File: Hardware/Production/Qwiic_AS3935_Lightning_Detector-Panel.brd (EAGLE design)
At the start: 123.2 x 123.2 mm, 1075 parts, among them U1 AS3935, U10 AS3935, U11 AS3935, U12 AS3935, U13 AS3935, U14 AS3935, U15 AS3935, U16 AS3935, U2 AS3935, U3 AS3935, U4 AS3935, U5 AS3935, U6 AS3935, U7 AS3935, U8 AS3935, U9 AS3935

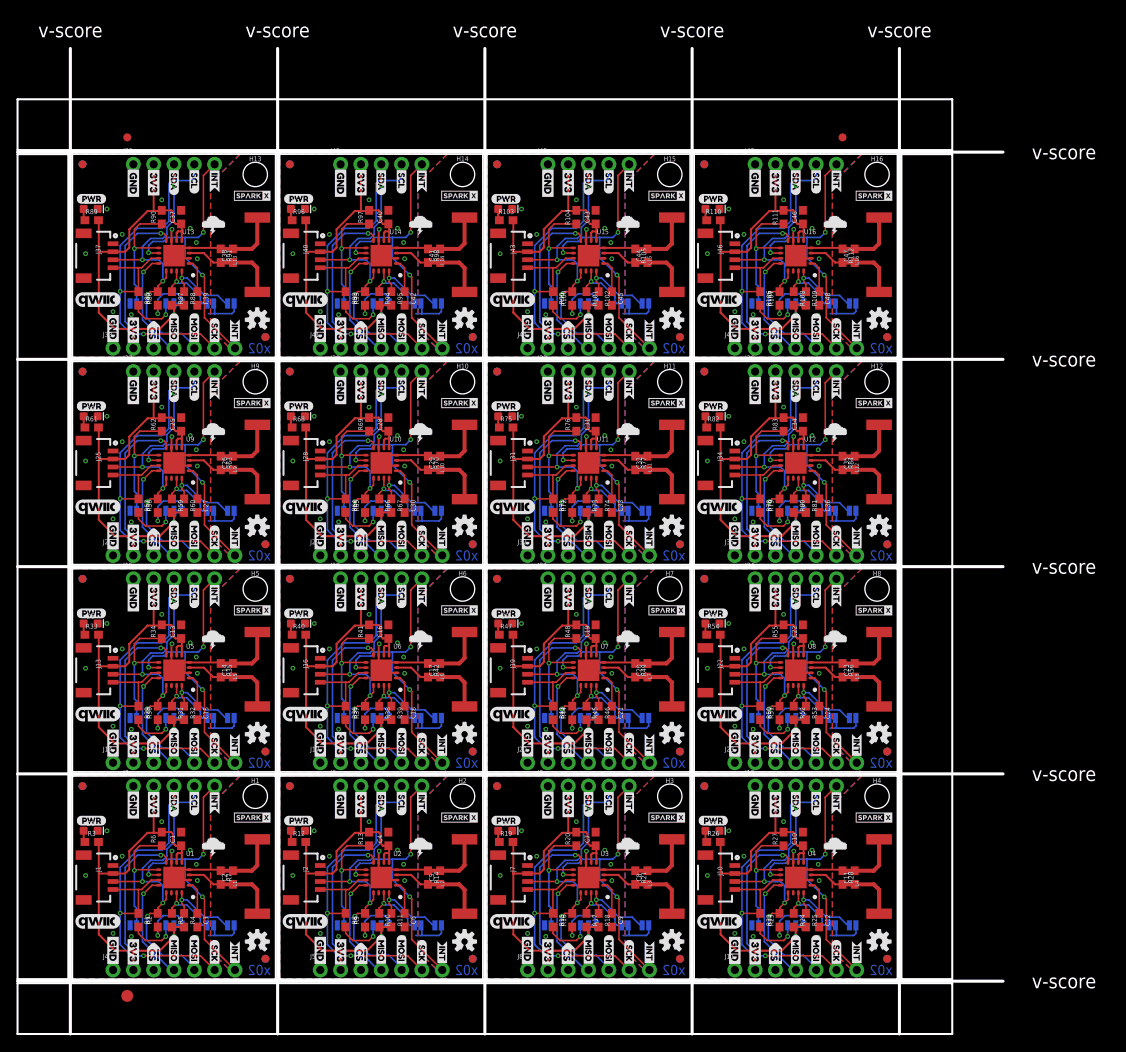
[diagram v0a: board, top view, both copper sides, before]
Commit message: One more time
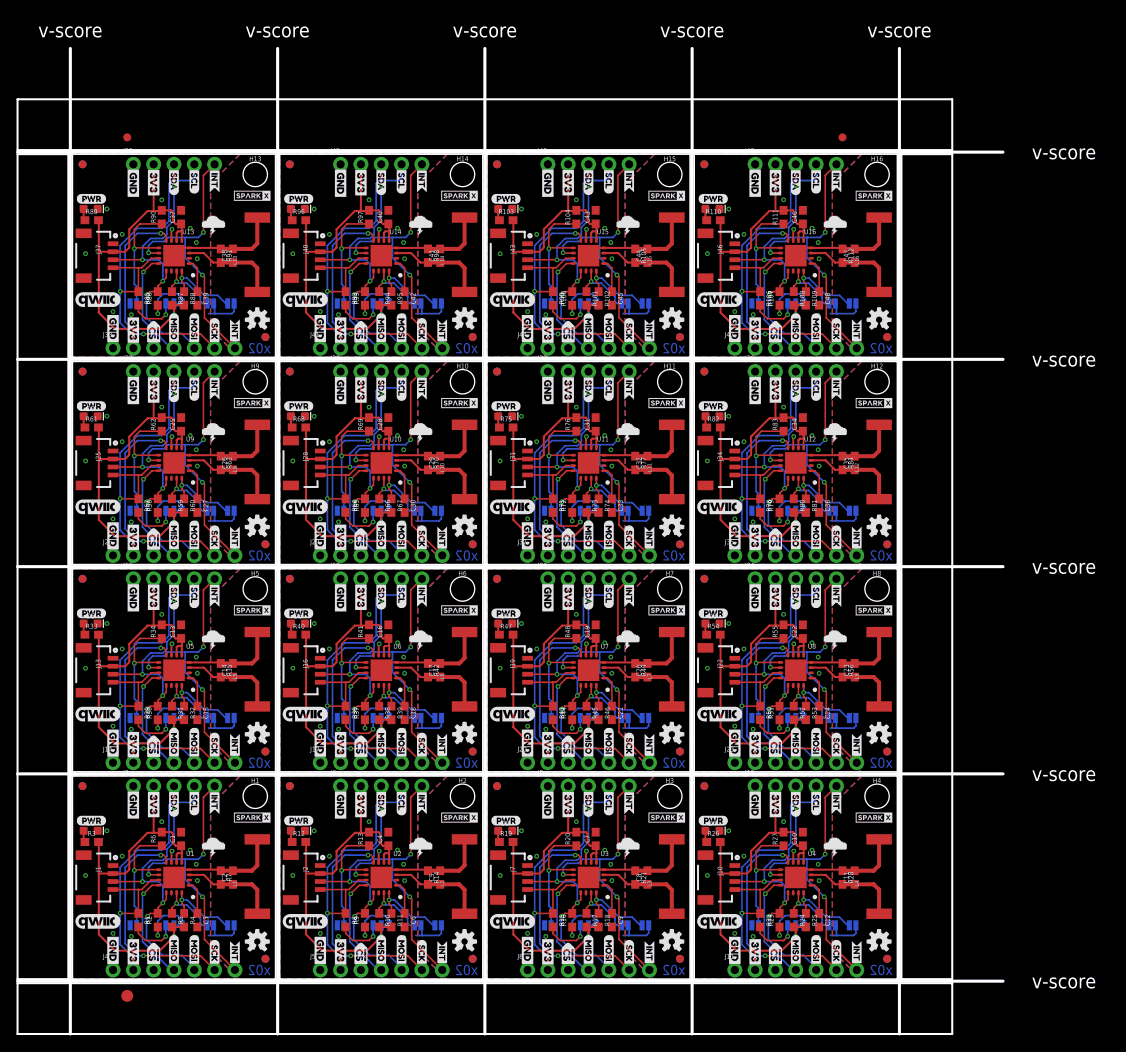
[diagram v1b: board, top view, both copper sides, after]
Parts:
- removed FRAME1, FRAME10, FRAME11, FRAME12, FRAME13, FRAME14, FRAME15, FRAME16, FRAME2, FRAME3, FRAME4, FRAME5, FRAME6, FRAME7, FRAME8, FRAME9: FRAME-LETTER, SparkFun-Aesthetics:CREATIVE_COMMONS
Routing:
- net GND7: track 25.6 -> 22.7 mm
- net GND6: track 25.6 -> 22.7 mm
- net GND5: track 25.6 -> 22.7 mm
- net GND4: track 25.6 -> 22.7 mm
- net GND3: track 25.6 -> 22.7 mm
- net GND2: track 25.6 -> 22.7 mm
- net GND1: track 25.6 -> 22.7 mm
- net GND: track 25.6 -> 22.7 mm
- net GND9: track 25.6 -> 22.7 mm
- net GND15: track 25.6 -> 22.7 mm
- net GND14: track 25.6 -> 22.7 mm
- net GND13: track 25.6 -> 22.7 mm
- net GND11: track 25.6 -> 22.7 mm
- net GND10: track 25.6 -> 22.7 mm
- net GND8: track 25.6 -> 22.7 mm
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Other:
- board text removed: "Elias Santistevan"
